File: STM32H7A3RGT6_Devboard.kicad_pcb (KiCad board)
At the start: 2 copper layers, 1 part, among them U1 STM32H7A3RGT6

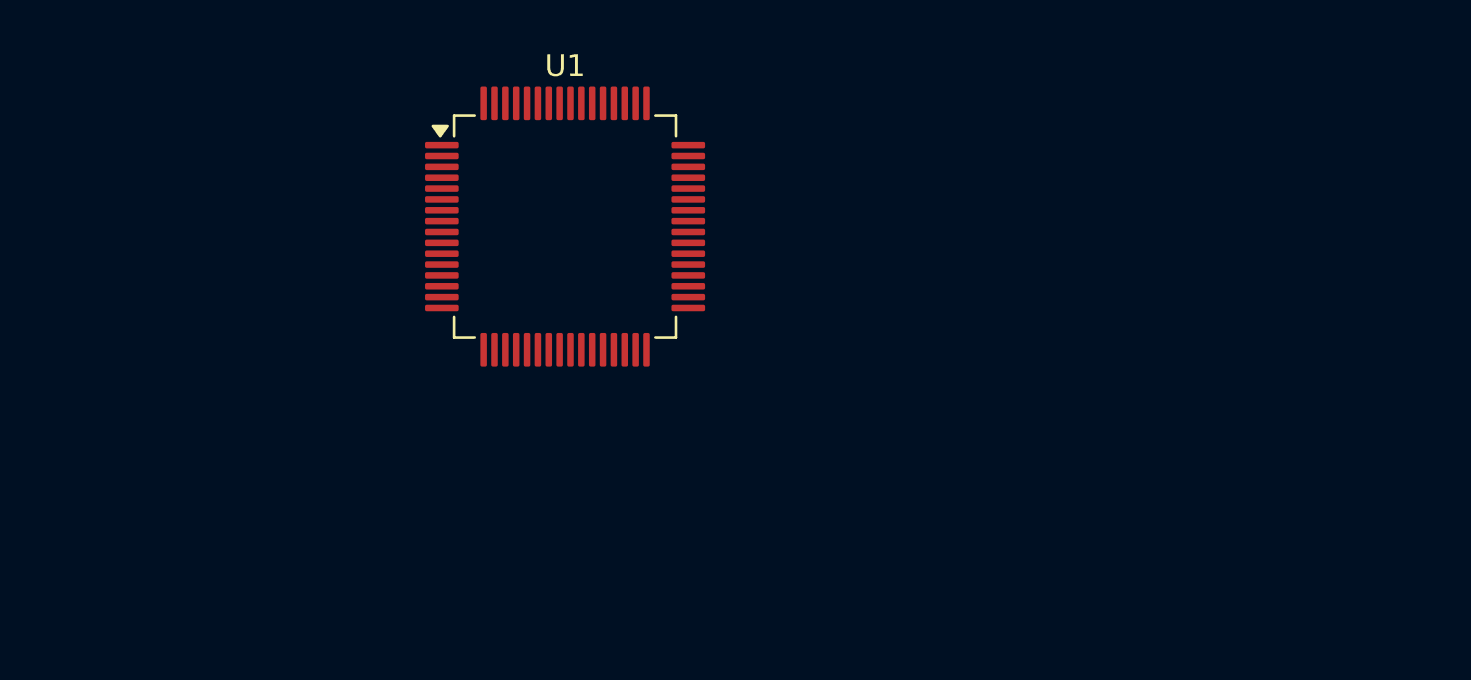
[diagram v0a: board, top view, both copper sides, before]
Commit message: First full draft
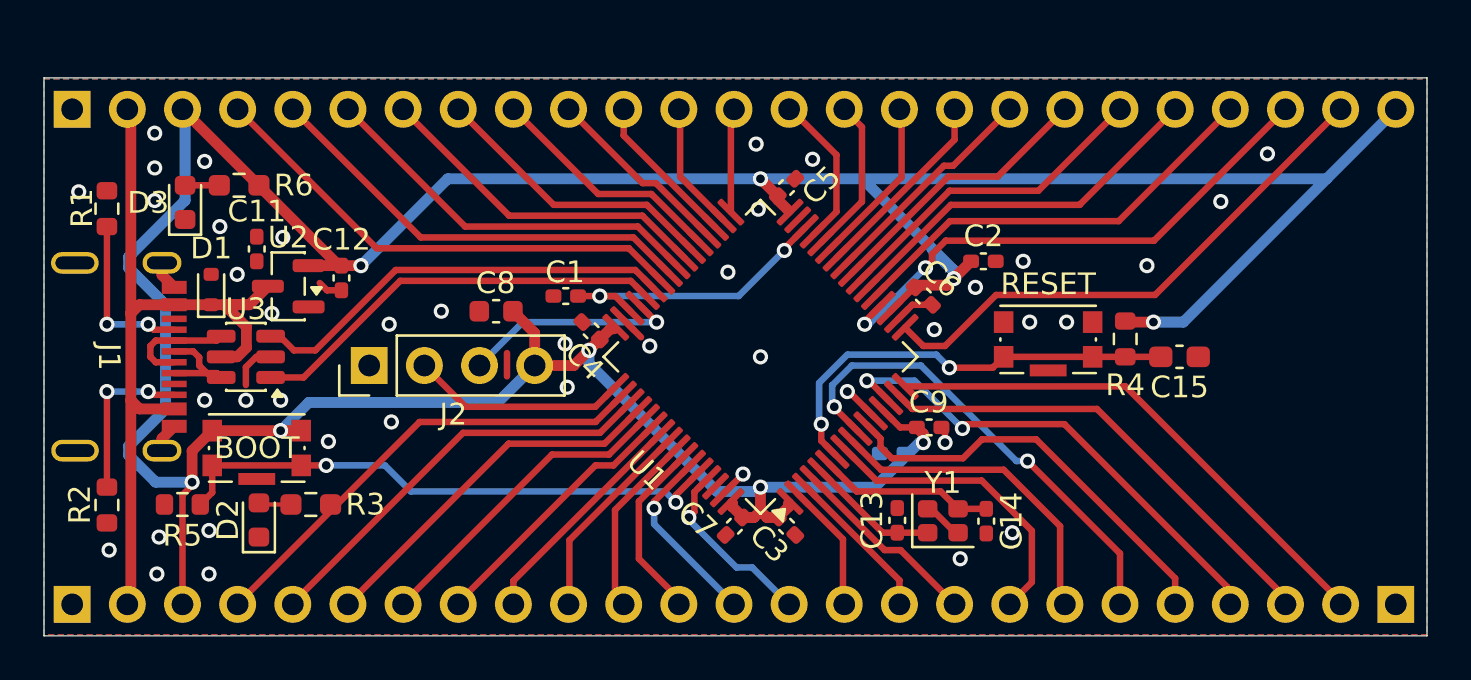
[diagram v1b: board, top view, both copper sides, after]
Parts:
- added C1: 2u2, Capacitor_SMD:C_0402_1005Metric_Pad0.74x0.62mm_HandSolder, F.Cu at (121.0, 97.2)
- added C10: 1u, Capacitor_SMD:C_0402_1005Metric_Pad0.74x0.62mm_HandSolder, B.Cu at (136.1, 104.5)
- added C11: 1uF, Capacitor_SMD:C_0402_1005Metric_Pad0.74x0.62mm_HandSolder, F.Cu at (106.8, 95.0)
- added C12: 1uF, Capacitor_SMD:C_0402_1005Metric_Pad0.74x0.62mm_HandSolder, F.Cu at (110.7, 96.4)
- added C13: 8pF, Capacitor_SMD:C_0402_1005Metric_Pad0.74x0.62mm_HandSolder, F.Cu at (136.3, 107.5)
- added C14: 8pF, Capacitor_SMD:C_0402_1005Metric_Pad0.74x0.62mm_HandSolder, F.Cu at (140.4, 107.6)
- added C15: 1uF, Capacitor_SMD:C_0603_1608Metric_Pad1.08x0.95mm_HandSolder, F.Cu at (149.3, 100.0)
- added C2: 1u, Capacitor_SMD:C_0402_1005Metric_Pad0.74x0.62mm_HandSolder, F.Cu at (140.3, 95.6)
- added C3: 100n, Capacitor_SMD:C_0402_1005Metric_Pad0.74x0.62mm_HandSolder, F.Cu at (131.2, 107.8)
- added C4: 100n, Capacitor_SMD:C_0402_1005Metric_Pad0.74x0.62mm_HandSolder, F.Cu at (122.2, 98.8)
- added C5: 100n, Capacitor_SMD:C_0402_1005Metric_Pad0.74x0.62mm_HandSolder, F.Cu at (131.2, 92.2)
- added C6: 100n, Capacitor_SMD:C_0402_1005Metric_Pad0.74x0.62mm_HandSolder, F.Cu at (137.5, 97.2)
- added C7: 100n, Capacitor_SMD:C_0402_1005Metric_Pad0.74x0.62mm_HandSolder, F.Cu at (128.8, 107.8)
- added C8: 4u7, Capacitor_SMD:C_0603_1608Metric, F.Cu at (117.8, 97.9)
- added C9: 100n, Capacitor_SMD:C_0402_1005Metric_Pad0.74x0.62mm_HandSolder, F.Cu at (137.8, 103.2)
- added D1: DF2B7AE, Diode_SMD:D_SOD-523, F.Cu at (104.7, 96.9)
- added D2: LED, LED_SMD:LED_0603_1608Metric, F.Cu at (106.9, 107.5)
- added D3: LED, LED_SMD:LED_0603_1608Metric, F.Cu at (103.5, 92.9)
- added J1: USB_C_Receptacle_USB2.0_14P, USBC:USB_C_Receptacle_Molex_217179-0001, F.Cu at (100.0, 100.0)
- added J2: Conn_01x04_Socket, Connector_PinHeader_2.54mm:PinHeader_1x04_P2.54mm_Vertical, F.Cu at (112.0, 100.4)
- added J3: Conn_01x25_PinHeader, Connector_PinHeader_2.54mm:PinHeader_1x25_P2.54mm_Vertical, B.Cu at (98.3, 88.6)
- added J4: Conn_01x25_PinHeader, Connector_PinHeader_2.54mm:PinHeader_1x25_P2.54mm_Vertical, B.Cu at (98.3, 111.4)
- added R1: 5k1, Resistor_SMD:R_0603_1608Metric, F.Cu at (99.9, 93.2)
- added R2: 5k1, Resistor_SMD:R_0603_1608Metric, F.Cu at (99.9, 106.8)
- added R3: 1k, Resistor_SMD:R_0603_1608Metric_Pad0.98x0.95mm_HandSolder, F.Cu at (109.3, 106.8)
- added R4: 5k1, Resistor_SMD:R_0603_1608Metric, F.Cu at (146.8, 99.2)
- added R5: 5k1, Resistor_SMD:R_0603_1608Metric, F.Cu at (103.4, 106.8)
- added R6: 1k, Resistor_SMD:R_0603_1608Metric_Pad0.98x0.95mm_HandSolder, F.Cu at (106.0, 92.1)
- added SW1: RESET, Button_Switch_SMD:SW_Push_1P1T-SH_NO_CK_KMR2xxG, F.Cu at (143.2, 99.2)
- added SW2: BOOT, Button_Switch_SMD:SW_Push_1P1T-SH_NO_CK_KMR2xxG, F.Cu at (106.8, 104.2)
- added U2: AP2127N-3.3TRG1, Package_TO_SOT_SMD:SOT-23, F.Cu at (108.2, 96.8)
- added U3: USBLC6-2SC6, Package_TO_SOT_SMD:SOT-23-6, F.Cu at (106.3, 100.0)
- added Y1: 12MHz, Crystal:Crystal_SMD_2016-4Pin_2.0x1.6mm, F.Cu at (138.4, 107.5)
- moved U1 10.8 mm to (130.0, 100.0), turned to 135 degrees
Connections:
- U1 pad 10: unconnected-(U1-PC2-Pad10) -> /PC2
- U1 pad 11: unconnected-(U1-PC3-Pad11) -> /PC3
- U1 pad 14: unconnected-(U1-PA0-Pad14) -> /PA0
- U1 pad 15: unconnected-(U1-PA1-Pad15) -> /PA1
- U1 pad 16: unconnected-(U1-PA2-Pad16) -> /PA2
- U1 pad 17: unconnected-(U1-PA3-Pad17) -> /PA3
- U1 pad 2: unconnected-(U1-PC13-Pad2) -> /PC13
- U1 pad 20: unconnected-(U1-PA4-Pad20) -> /PA4
- U1 pad 21: unconnected-(U1-PA5-Pad21) -> /PA5
- U1 pad 22: unconnected-(U1-PA6-Pad22) -> /PA6
- U1 pad 23: unconnected-(U1-PA7-Pad23) -> /PA7
- U1 pad 24: unconnected-(U1-PC4-Pad24) -> /PC4
- U1 pad 25: unconnected-(U1-PC5-Pad25) -> /PC5
- U1 pad 26: unconnected-(U1-PB0-Pad26) -> /PB0
- U1 pad 27: unconnected-(U1-PB1-Pad27) -> /PB1
- U1 pad 28: unconnected-(U1-PB2-Pad28) -> /PB2
- U1 pad 29: unconnected-(U1-PB10-Pad29) -> /PB10
- U1 pad 3: unconnected-(U1-PC14-Pad3) -> /PC14
- U1 pad 33: unconnected-(U1-PB12-Pad33) -> /PB12
- U1 pad 34: unconnected-(U1-PB13-Pad34) -> /PB13
- U1 pad 35: unconnected-(U1-PB14-Pad35) -> /PB14
- U1 pad 36: unconnected-(U1-PB15-Pad36) -> /PB15
- U1 pad 37: unconnected-(U1-PC6-Pad37) -> /PC6
- U1 pad 38: unconnected-(U1-PC7-Pad38) -> /PC7
- U1 pad 39: unconnected-(U1-PC9-Pad39) -> /PC9
- U1 pad 4: unconnected-(U1-PC15-Pad4) -> /PC15
- U1 pad 40: unconnected-(U1-PA8-Pad40) -> /PA8
- U1 pad 41: unconnected-(U1-PA9-Pad41) -> /PA9
- U1 pad 42: unconnected-(U1-PA10-Pad42) -> /PA10
- U1 pad 43: unconnected-(U1-PA11-Pad43) -> /USB_D-
- U1 pad 44: unconnected-(U1-PA12-Pad44) -> /USB_D+
- U1 pad 45: unconnected-(U1-PA13-Pad45) -> /SWDIO
- U1 pad 49: unconnected-(U1-PA14-Pad49) -> /SWCLK
- U1 pad 5: unconnected-(U1-PH0-Pad5) -> /OSC_IN
- U1 pad 50: unconnected-(U1-PA15-Pad50) -> /PA15
- U1 pad 51: unconnected-(U1-PC10-Pad51) -> /PC10
- U1 pad 52: unconnected-(U1-PC11-Pad52) -> /PC11
- U1 pad 53: unconnected-(U1-PC12-Pad53) -> /PC12
- U1 pad 54: unconnected-(U1-PD2-Pad54) -> /PD2
- U1 pad 55: unconnected-(U1-PB3-Pad55) -> /PB3
- U1 pad 56: unconnected-(U1-PB4-Pad56) -> /PB4
- U1 pad 57: unconnected-(U1-PB5-Pad57) -> /PB5
- U1 pad 58: unconnected-(U1-PB6-Pad58) -> /PB6
- U1 pad 59: unconnected-(U1-PB7-Pad59) -> /PB7
- U1 pad 6: unconnected-(U1-PH1-Pad6) -> /OSC_OUT
- U1 pad 61: unconnected-(U1-PB8-Pad61) -> /PB8
- U1 pad 62: unconnected-(U1-PB9-Pad62) -> /PB9
- U1 pad 8: unconnected-(U1-PC0-Pad8) -> /PC0
- U1 pad 9: unconnected-(U1-PC1-Pad9) -> /PC1
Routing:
- net +3V3: track 0.00 -> 172.0 mm, vias 0 -> 9
- net VBUS: track 0.00 -> 36.8 mm
- net /BOOT0: track 0.00 -> 25.5 mm, vias 0 -> 2
- net /PA3: track 0.00 -> 24.9 mm
- net /PA4: track 0.00 -> 24.9 mm, vias 0 -> 2
- net /PA2: track 0.00 -> 24.3 mm
- net /PA0: track 0.00 -> 23.0 mm, vias 0 -> 2
- net /PA10: track 0.00 -> 22.8 mm
- net /PC2: track 0.00 -> 22.3 mm, vias 0 -> 2
- net /PA1: track 0.00 -> 22.1 mm
- net /PA15: track 0.00 -> 21.8 mm
- net /PA9: track 0.00 -> 20.5 mm
- net /NRST: track 0.00 -> 20.4 mm, vias 0 -> 2
- net /PA5: track 0.00 -> 20.0 mm
- net /USB_D-: track 0.00 -> 19.8 mm
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- added copper zone on B.Cu, net GND
- added copper zone on F.Cu, net GND
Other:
- board outline added: 63.7 x 25.7 mm
